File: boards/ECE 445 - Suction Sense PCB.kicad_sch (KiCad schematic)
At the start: 12 parts, among them U1 ESP32-WROOM-32E, U2 TPS2120YFPR, U3 AP62150Z6

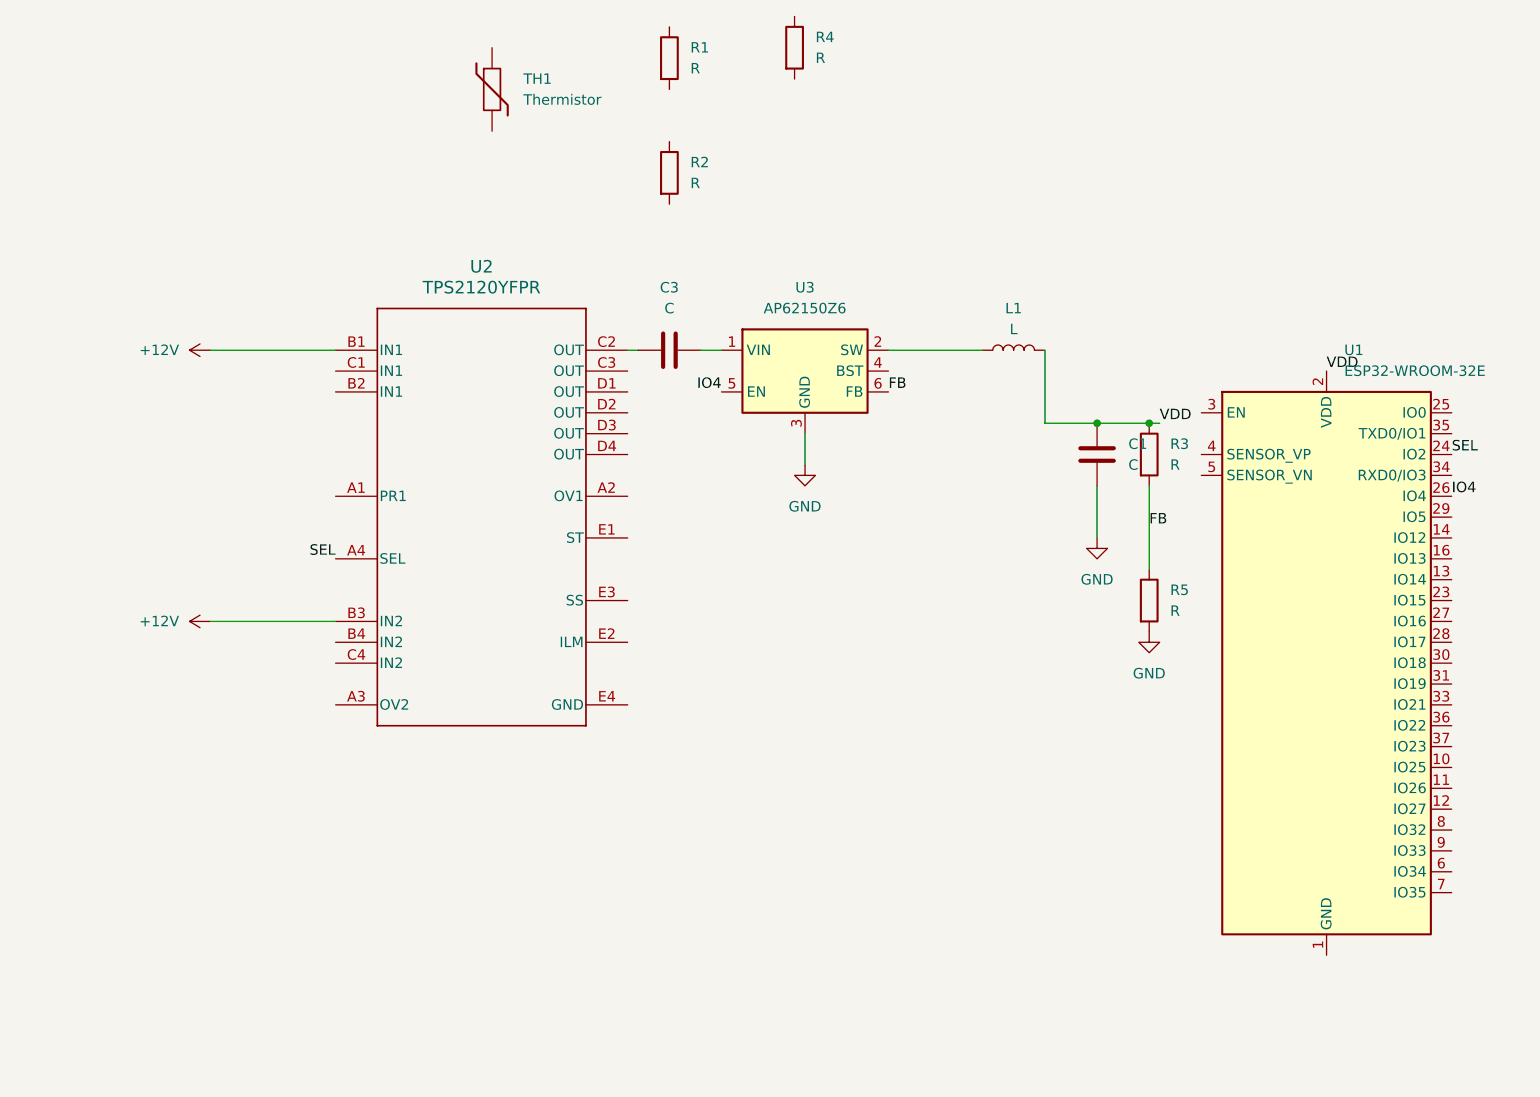
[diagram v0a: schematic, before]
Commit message: finished buck
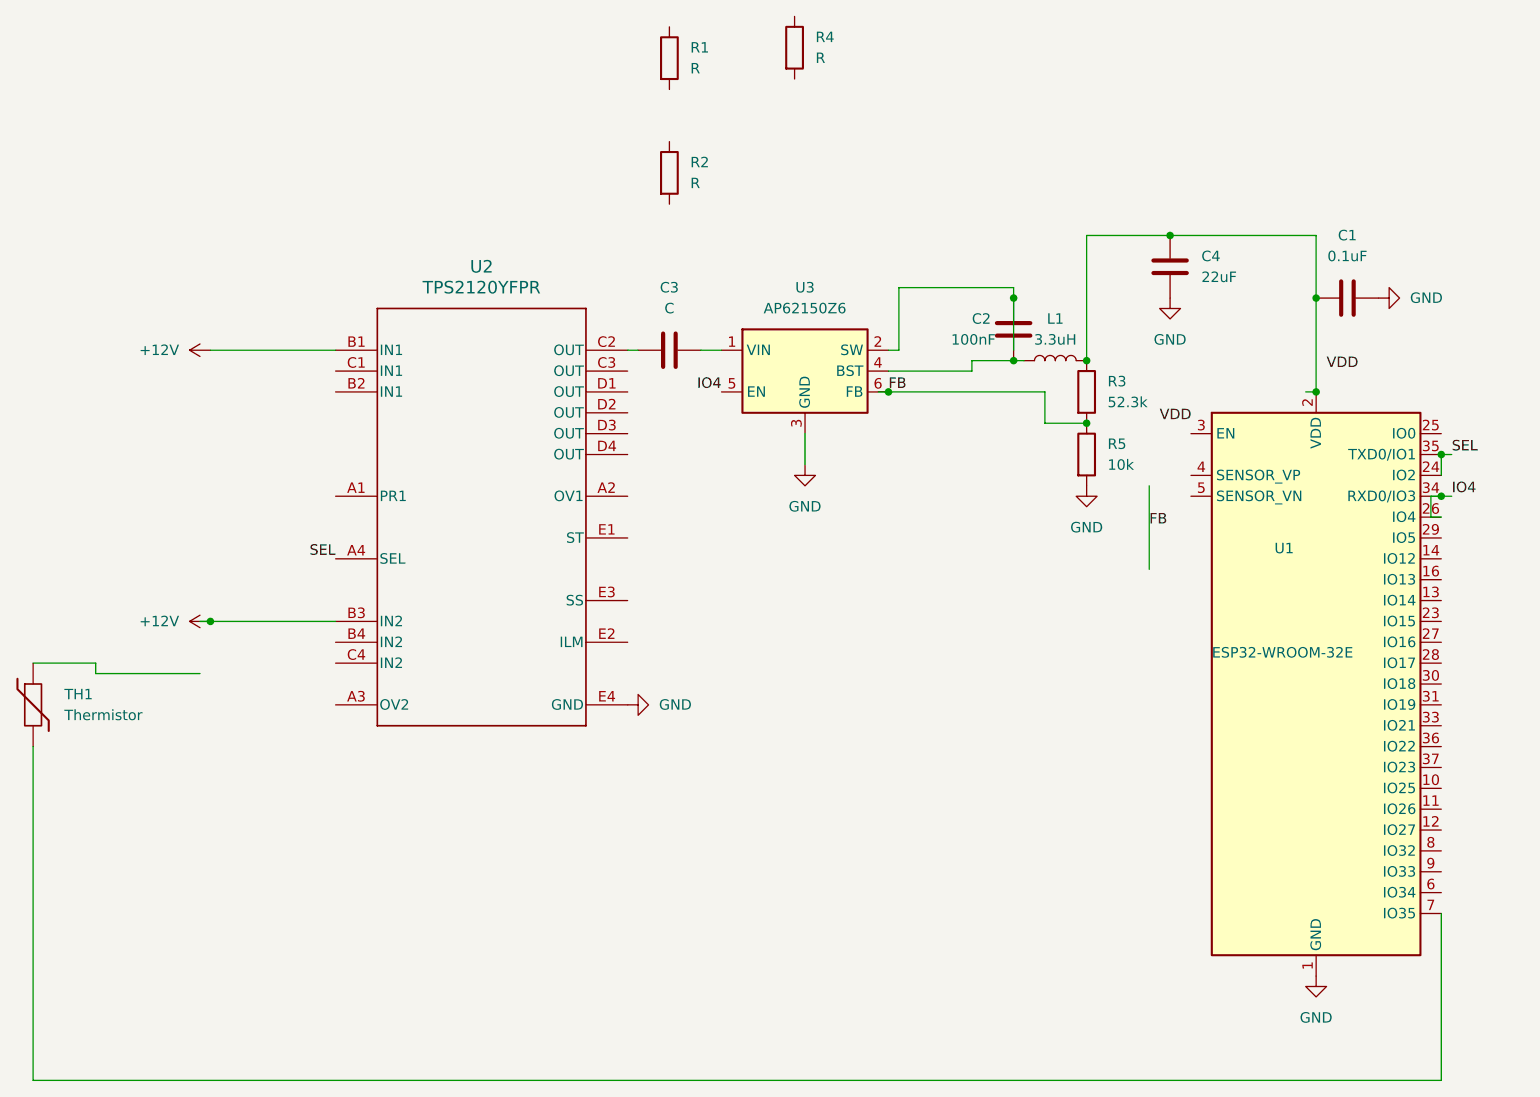
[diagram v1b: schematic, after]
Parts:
- added C2: 100nF, symbol Device:C
- added C4: 22uF, symbol Device:C
- C1: value C -> 0.1uF
- L1: value L -> 3.3uH
- R3: value R -> 52.3k
- R5: value R -> 10k
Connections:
- net GND: now also C1.2, U1.1 (GND), U1.15 (GND), U1.38 (GND), U1.39 (GND), U2.E4 (GND), C4.2; no longer C1.1
- net IO4: now also U1.34 (RXD0/IO3)
- net SEL: now also U1.35 (TXD0/IO1)
- net VDD: no longer C1.2, L1.2, R3.1, U1.2 (VDD)
- net at L1.1: now also U3.4 (BST), C2.2; no longer U3.2 (SW)
- net at TH1.2: now also U1.7 (IO35)
- new net: C1.1, C4.1, L1.2, R3.1, U1.2 (VDD)
- new net: C2.1, U3.2 (SW)
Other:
- moved on the sheet: C1, TH1, U1
